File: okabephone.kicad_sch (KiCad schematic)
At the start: 49 parts, among them J1 Micro_SD_Card_Det1, J6 SFH11-PBPC-D10-RA-BK, M1 Motor_DC, Q1 AO3400A, SW1 SW_Push, SW10 SW_Push, SW11 SW_Push, SW12 SW_Push, SW13 SW_Push, SW14 SW_Push, SW15 SW_Push, SW16 SW_Push, SW17 SW_Push, SW18 SW_Push, SW19 SW_Push, SW2 SW_Push, SW21 SW_Push, SW3 SW_Push, SW4 SW_Push, SW5 SW_Push, SW6 SW_Push, SW7 SW_Push, SW8 SW_Push, SW9 SW_Push, U1 MCP23017_ML, U2 ESP32-S3-WROOM-1, U6 PCF8563T, Y1 32.768kHz

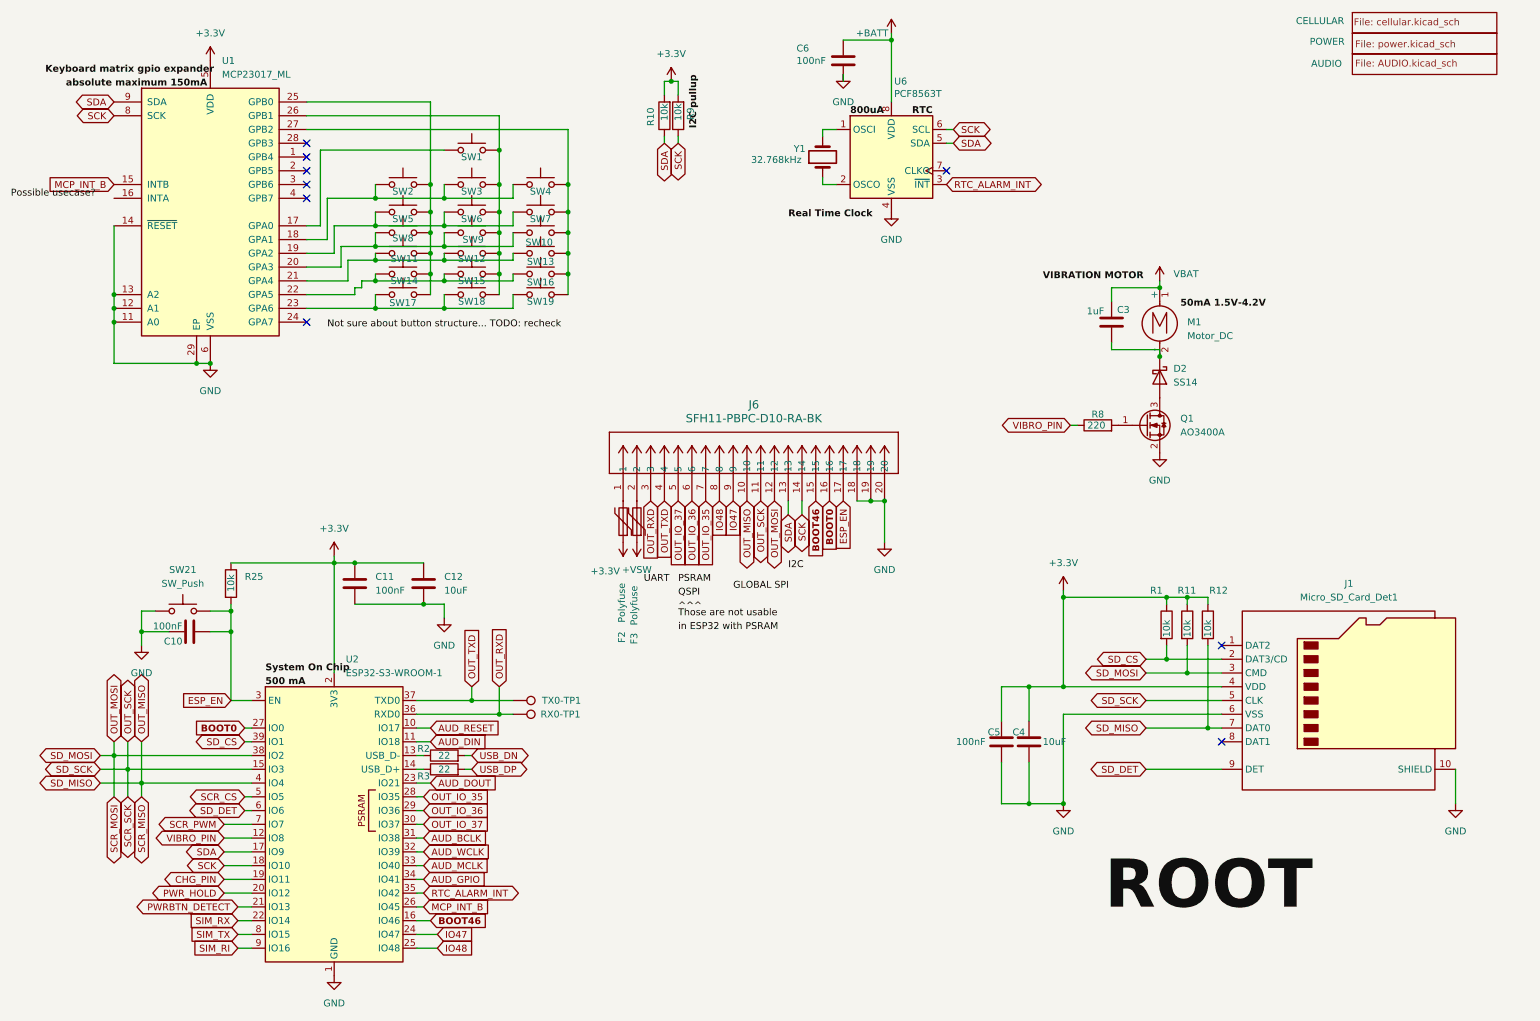
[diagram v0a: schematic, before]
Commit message: mblya
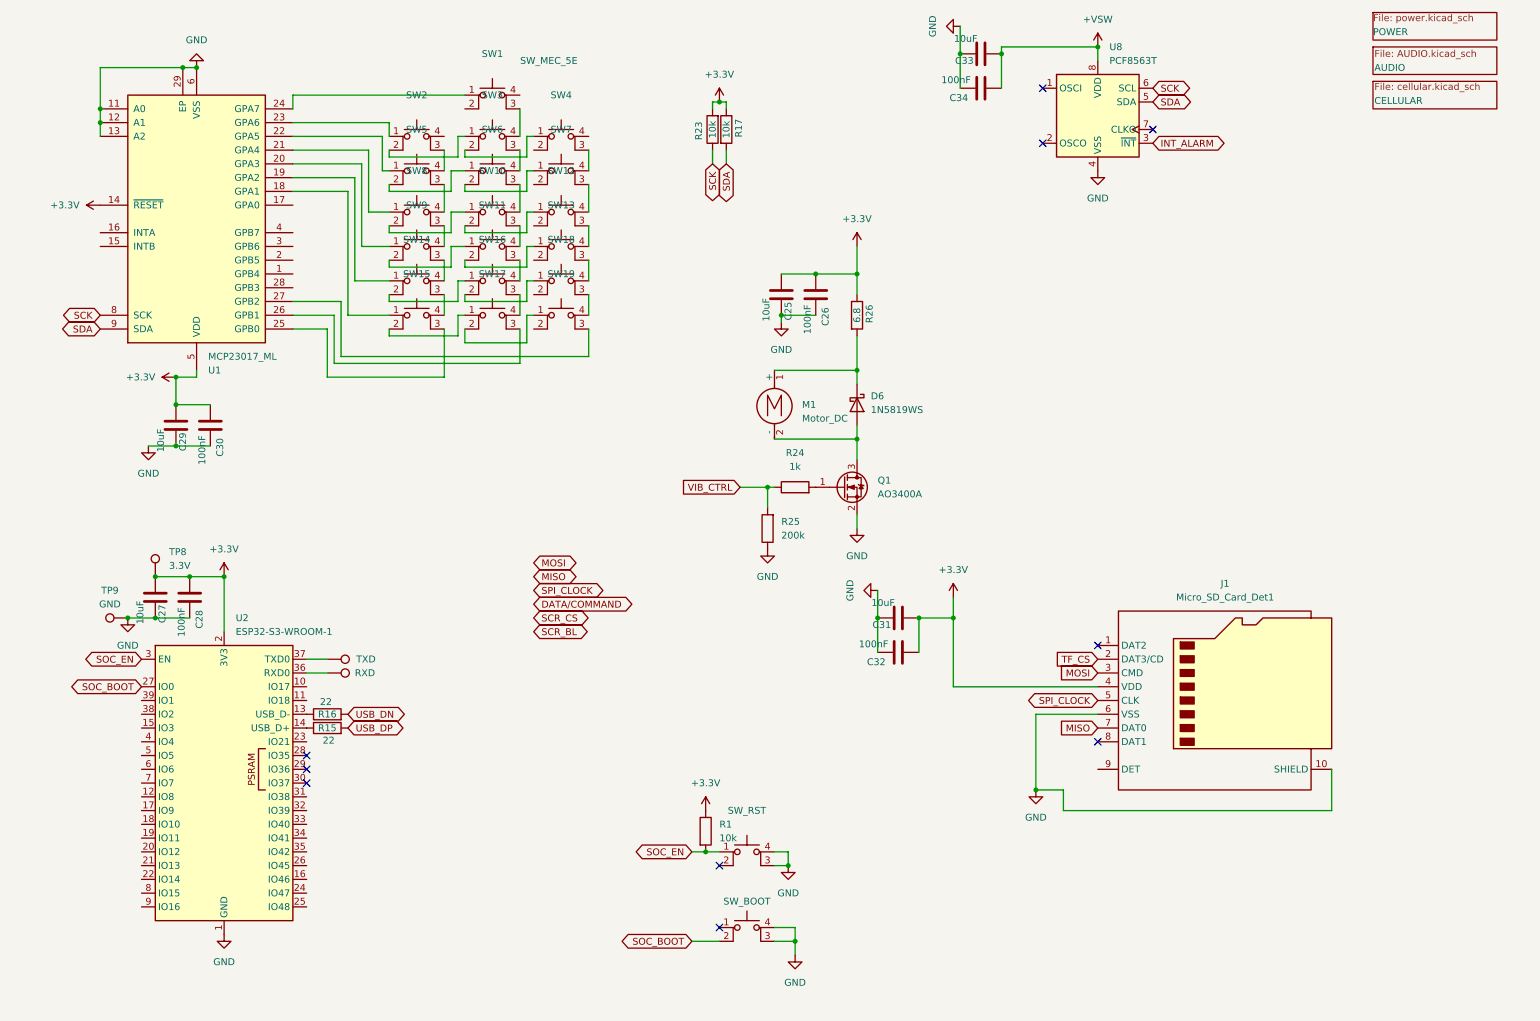
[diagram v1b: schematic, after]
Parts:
- removed C10, C11, C5, C6: 100nF, symbol Device:C
- removed C12, C4: 10uF, symbol Device:C
- removed C3: 1uF, symbol Device:C
- removed D2: SS14, Diode_SMD:D_SMA, symbol Diode:SS14
- removed F2, F3: Polyfuse, symbol Device:Polyfuse
- removed J6: SFH11-PBPC-D10-RA-BK, connector:CONN20_D10-RA-BK_SUL, symbol 20PIN Connector:SFH11-PBPC-D10-RA-BK
- removed R10, R11, R12, R9: 10k, symbol Device:R
- removed R2, R3: 22, symbol Device:R
- removed R8: 220, symbol Device:R
- removed RX0-TP1, TX0-TP1: TestPoint, symbol Connector:TestPoint
- removed SW1, SW10, SW11, SW12, SW13, SW14, SW15, SW16, SW17, SW18, SW19, SW2, SW21, SW3, SW4, SW5, SW6, SW7, SW8, SW9: SW_Push, symbol Switch:SW_Push
- removed U6: PCF8563T, Package_SO:SOIC-8_3.9x4.9mm_P1.27mm, symbol Timer_RTC:PCF8563T
- removed Y1: 32.768kHz, Crystal:Crystal_SMD_3215-2Pin_3.2x1.5mm, symbol Device:Crystal
- added C25, C27, C29, C31, C33: 10uF, symbol Device:C
- added C26, C28, C30, C32, C34: 100nF, symbol Device:C
- added D6: 1N5819WS, Diode_SMD:D_SOD-323, symbol Diode:1N5819WS
- added R15, R16: 22, symbol Device:R
- added R17, R23: 10k, symbol Device:R
- added R24: 1k, symbol Device:R
- added R26: 6.8, symbol Device:R
- added RXD, TXD: TestPoint, symbol Connector:TestPoint
- added SW1, SW10, SW11, SW12, SW13, SW14, SW15, SW16, SW17, SW18, SW19, SW2, SW3, SW4, SW5, SW6, SW7, SW8, SW9, SW_BOOT, SW_RST: SW_MEC_5E, symbol Switch:SW_MEC_5E
- added TP8: 3.3V, symbol Connector:TestPoint
- added TP9: GND, symbol Connector:TestPoint
- added U8: PCF8563T, Package_SO:SOIC-8_3.9x4.9mm_P1.27mm, symbol Timer_RTC:PCF8563T
- R25: value 10k -> 200k
- U2: footprint RF_Module:ESP32-S3-WROOM-1U -> RF_Module:ESP32-S3-WROOM-1
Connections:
- net +3.3V: now also U1.14 (~{RESET}), C25.2, C26.2, C27.2, C28.2, C29.2, C30.2, C31.2, C32.2, R17.1, R23.2, R26.1, TP8.1; no longer R25.1
- net +VSW: now also C33.2, C34.2, U8.8 (VDD)
- net GND: now also R25.1, C25.1, C26.1, C27.1, C28.1, C29.1, C30.1, C31.1, C32.1, C33.1, C34.1, SW_BOOT.3 (K), SW_BOOT.4 (A), SW_RST.3 (K), SW_RST.4 (A), TP9.1, U8.4 (VSS); no longer U1.14 (~{RESET})
- net SCK: now also R23.1, U8.6 (SCL); no longer U2.18 (IO10)
- net SCR_CS: no longer U2.5 (IO5)
- net SDA: now also R17.2, U8.5 (SDA); no longer U2.17 (IO9)
- net USB_DN: now also R16.2
- net USB_DP: now also R15.2
- net at M1.2 (-): now also Q1.3 (D), D6.2 (A)
- net at U1.19 (GPA2): now also SW14.1
- net at U1.27 (GPB2): now also SW19.3 (K)
- net at U2.13 (USB_D-): now also R16.1
- net at U2.14 (USB_D+): now also R15.1
- net at U1.21 (GPA4): now also SW8.1
- net at Q1.1 (G): now also R24.2
- net at U1.25 (GPB0): now also SW15.3 (K)
- net at U1.26 (GPB1): now also SW17.3 (K)
- net at U1.18 (GPA1): now also SW15.1
- net at U1.20 (GPA3): now also SW9.1
- net at U1.22 (GPA5): now also SW5.1
- net at U1.23 (GPA6): now also SW2.1
- net at U1.24 (GPA7): now also SW1.1
- net AUD_BCLK: no longer names the net of U2.31 (IO38)
- net AUD_DIN: no longer names the net of U2.11 (IO18)
- net AUD_DOUT: no longer names the net of U2.23 (IO21)
- net AUD_GPIO: no longer names the net of U2.34 (IO41)
- net AUD_MCLK: no longer names the net of U2.33 (IO40)
- net AUD_RESET: no longer names the net of U2.10 (IO17)
- net AUD_WCLK: no longer names the net of U2.32 (IO39)
- net BOOT0 renamed SOC_BOOT
- net SOC_BOOT: now also SW_BOOT.2
- net BOOT46: no longer names the net of U2.16 (IO46)
- net CHG_PIN: no longer names the net of U2.19 (IO11)
- net ESP_EN renamed SOC_EN
- net SOC_EN: now also R1.2, SW_RST.1; no longer R25.2
- net IO47: no longer names the net of U2.24 (IO47)
- net IO48: no longer names the net of U2.25 (IO48)
- net MCP_INT_B: no longer names the net of U2.26 (IO45)
- net MCP_INT_B: no longer U1.15 (INTB)
- net OUT_IO_35: no longer names the net of U2.28 (IO35)
- net OUT_IO_36: no longer names the net of U2.29 (IO36)
- net OUT_IO_37: no longer names the net of U2.30 (IO37)
- net OUT_MISO: no longer names the net of U2.4 (IO4)
- net OUT_MISO: no longer J1.7 (DAT0)
- net OUT_MOSI: no longer names the net of U2.38 (IO2)
- net OUT_MOSI: no longer J1.3 (CMD)
- net OUT_RXD: no longer names the net of U2.36 (RXD0)
- net OUT_RXD: now also RXD.1
- net OUT_SCK: no longer names the net of U2.15 (IO3)
- net OUT_SCK: no longer J1.5 (CLK)
- net OUT_TXD: no longer names the net of U2.37 (TXD0)
- net OUT_TXD: now also TXD.1
- net PWRBTN_DETECT: no longer names the net of U2.21 (IO13)
- net PWR_HOLD: no longer names the net of U2.20 (IO12)
- net RTC_ALARM_INT: no longer names the net of U2.35 (IO42)
- net SCR_PWM: no longer names the net of U2.7 (IO7)
- removed net SD_CS: J1.2 (DAT3/CD), R1.2, U2.39 (IO1)
- net SD_DET: no longer names the net of U2.6 (IO6)
- net SD_DET: no longer J1.9 (DET)
- net SIM_RI: no longer names the net of U2.9 (IO16)
- net SIM_RX: no longer names the net of U2.22 (IO14)
- net SIM_TX: no longer names the net of U2.8 (IO15)
- net VBAT: no longer names the net of M1.1 (+)
- net VBAT: now also D6.1 (K), R26.2
- net VIBRO_PIN: no longer names the net of U2.12 (IO8)
- new net: SW5.2, SW6.1
- new net: SW5.3 (K), SW8.4 (A)
- new net: SW2.3 (K), SW5.4 (A)
- new net: SW10.1, SW8.2
- new net: SW8.3 (K), SW9.4 (A)
- new net: SW15.2, SW17.1
- new net: SW14.3 (K), SW15.4 (A)
- new net: SW3.2, SW4.1
- new net: SW4.3 (K), SW7.4 (A)
- new net: SW1.3 (K), SW3.4 (A)
- new net: SW10.2, SW12.1
- new net: SW12.3 (K), SW13.4 (A)
- new net: SW12.4 (A), SW7.3 (K)
- new net: SW14.2, SW16.1
- new net: SW16.2, SW18.1
- new net: SW16.3 (K), SW17.4 (A)
- new net: SW11.3 (K), SW16.4 (A)
- new net: SW11.2, SW13.1
- new net: SW13.3 (K), SW18.4 (A)
- new net: SW6.2, SW7.1
- new net: SW11.1, SW9.2
- new net: SW10.3 (K), SW11.4 (A)
- new net: SW2.2, SW3.1
- new net: SW14.4 (A), SW9.3 (K)
- new net: SW3.3 (K), SW6.4 (A)
- new net: SW10.4 (A), SW6.3 (K)
- new net: SW17.2, SW19.1
- new net: SW18.3 (K), SW19.4 (A)
- new net INT_ALARM: U8.3 (~{INT})
- new net MISO: J1.7 (DAT0)
- new net MOSI: J1.3 (CMD)
- new net SPI_CLOCK: J1.5 (CLK)
- new net TF_CS: J1.2 (DAT3/CD)
- new net VIB_CTRL: R24.1, R25.2
- no-connect marks 9 -> 10
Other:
- company: Nergon -> (none)
- title: Okabe_Phone -> (none)
- moved on the sheet: J1, M1, U1, U2
